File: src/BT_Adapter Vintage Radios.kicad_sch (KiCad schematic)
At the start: 14 parts, among them J1 1V2_SEPARATED, J2 BT_VCC, J3 BT_GND, Q1 IRF620N, U1 PS2561, U2 LM7805

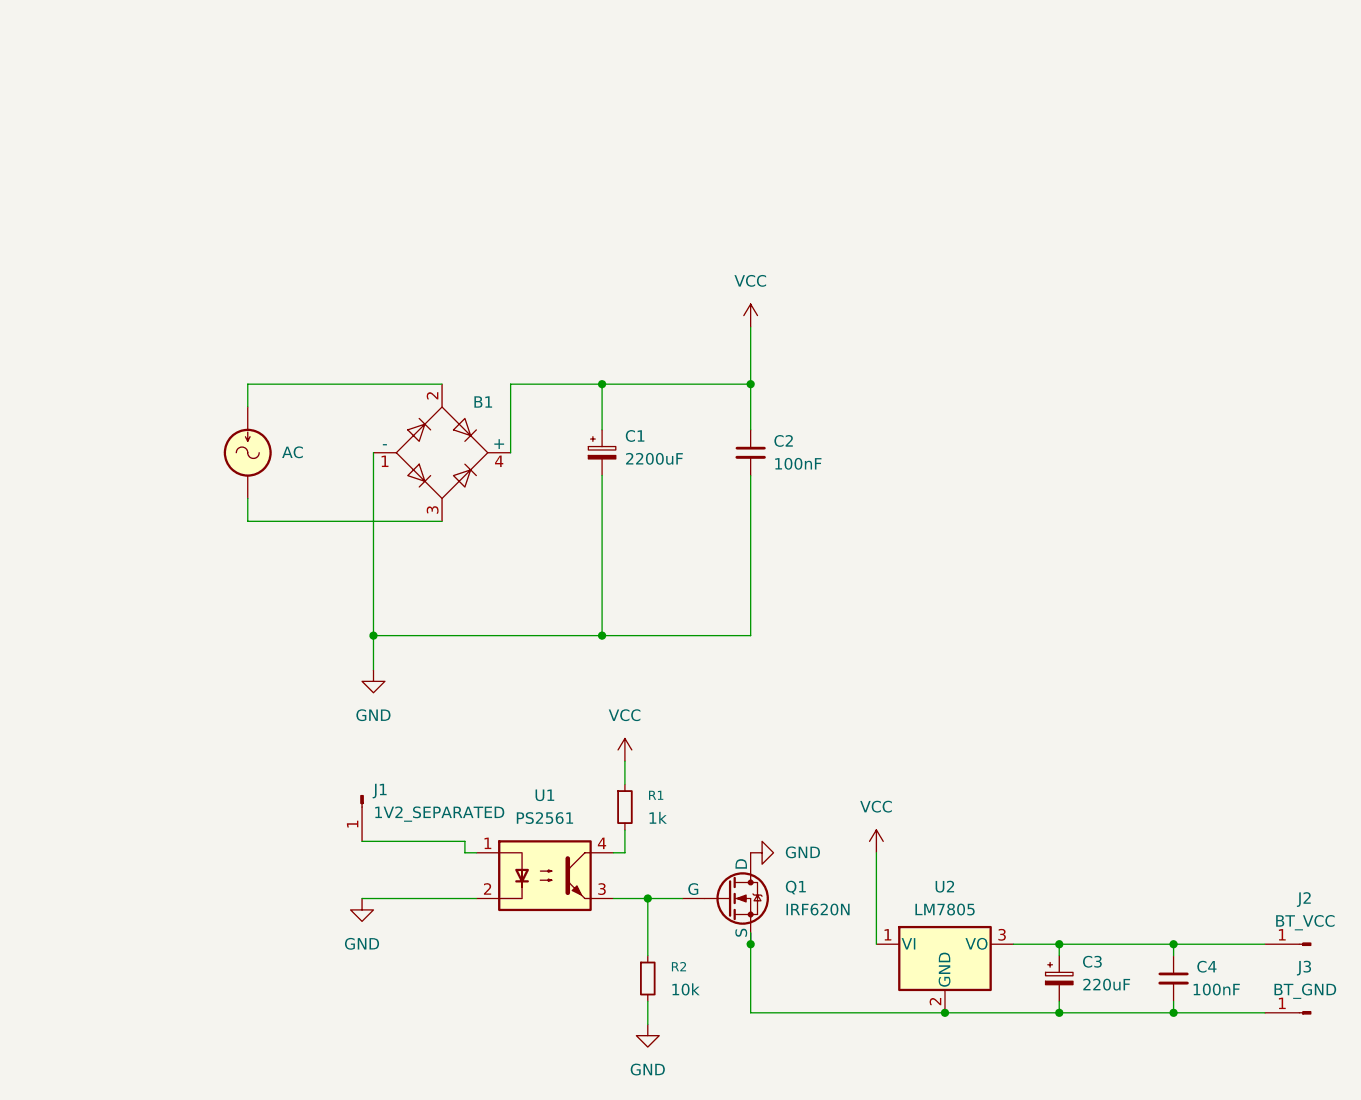
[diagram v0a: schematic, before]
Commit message: Minor improvements
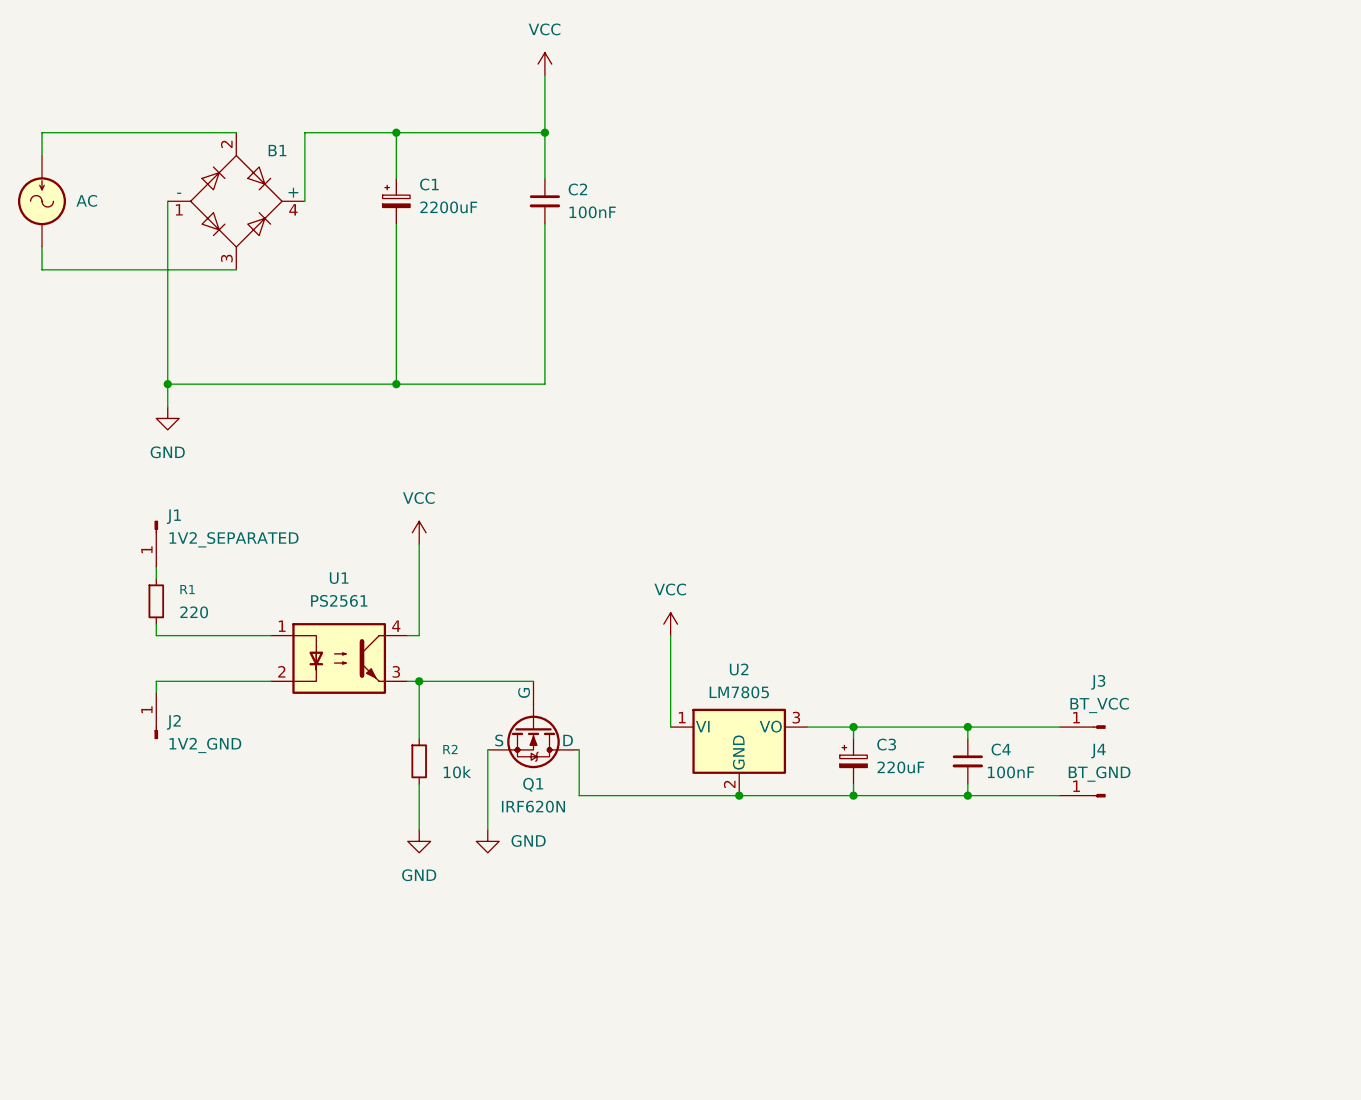
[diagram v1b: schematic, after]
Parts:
- added J2: 1V2_GND, Connector_Wire:SolderWire-0.1sqmm_1x01_D0.4mm_OD1mm, symbol Connector:Conn_01x01_Pin
- R1: value 1k -> 220
- renumbered J2 to J3, J3 to J4
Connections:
- net GND: now also Q1.3 (S); no longer Q1.1 (D), U1.2
- net VCC: now also U1.4; no longer R1.1
- net at R1.2: now also U1.1; no longer U1.4
- net at J1.1 (Pin_1): now also R1.1; no longer U1.1
- net at C3.2, C4.2, J4.1 (Pin_1)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: now also Q1.1 (D); no longer Q1.3 (S)
- new net: J2.1 (Pin_1), U1.2
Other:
- moved on the sheet: B1, C1, C2, C3, C4, J1, J3, J4, Q1, R2, U1, U2
